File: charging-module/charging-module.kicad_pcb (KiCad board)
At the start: 2 copper layers, 99 x 48 mm, 23 parts, among them IC1 MCP73871-2CCI_ML, J1 OUT, J2 USB_C_Receptacle_USB2.0_16P, J3 BAT

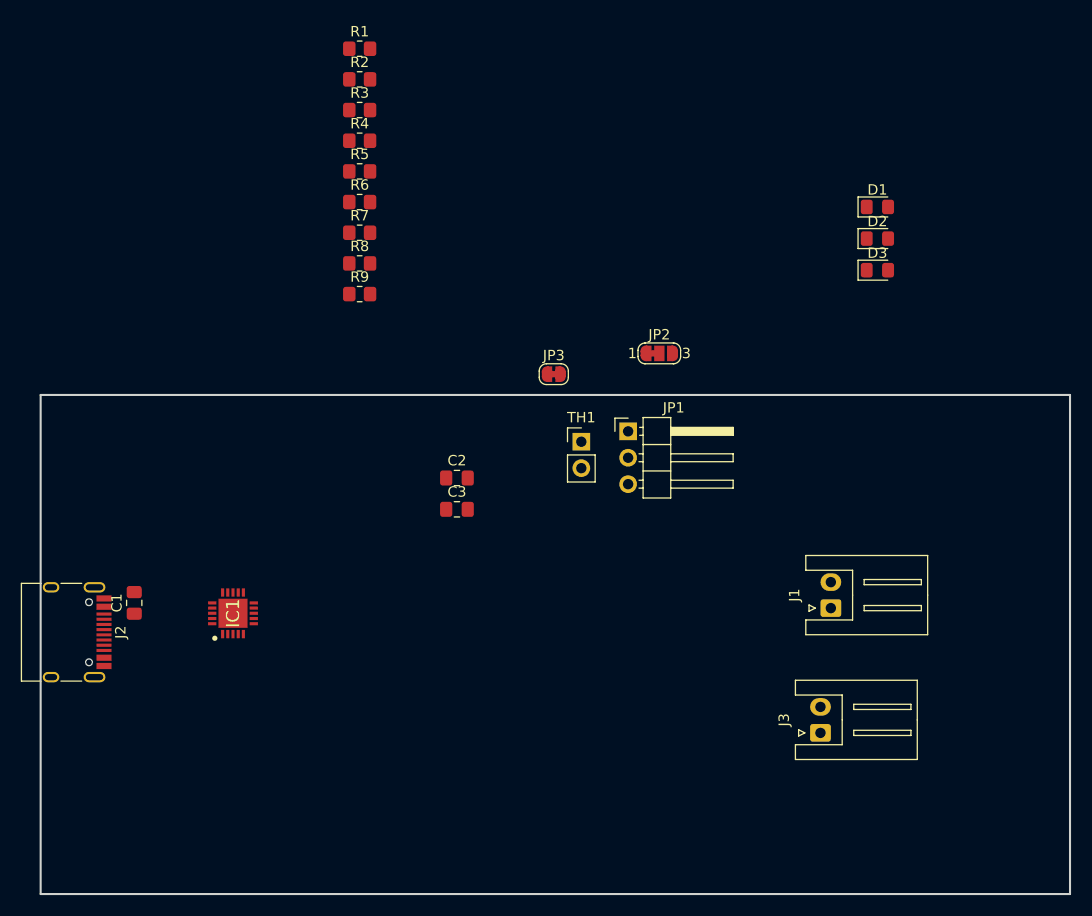
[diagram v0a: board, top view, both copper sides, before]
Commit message: layout
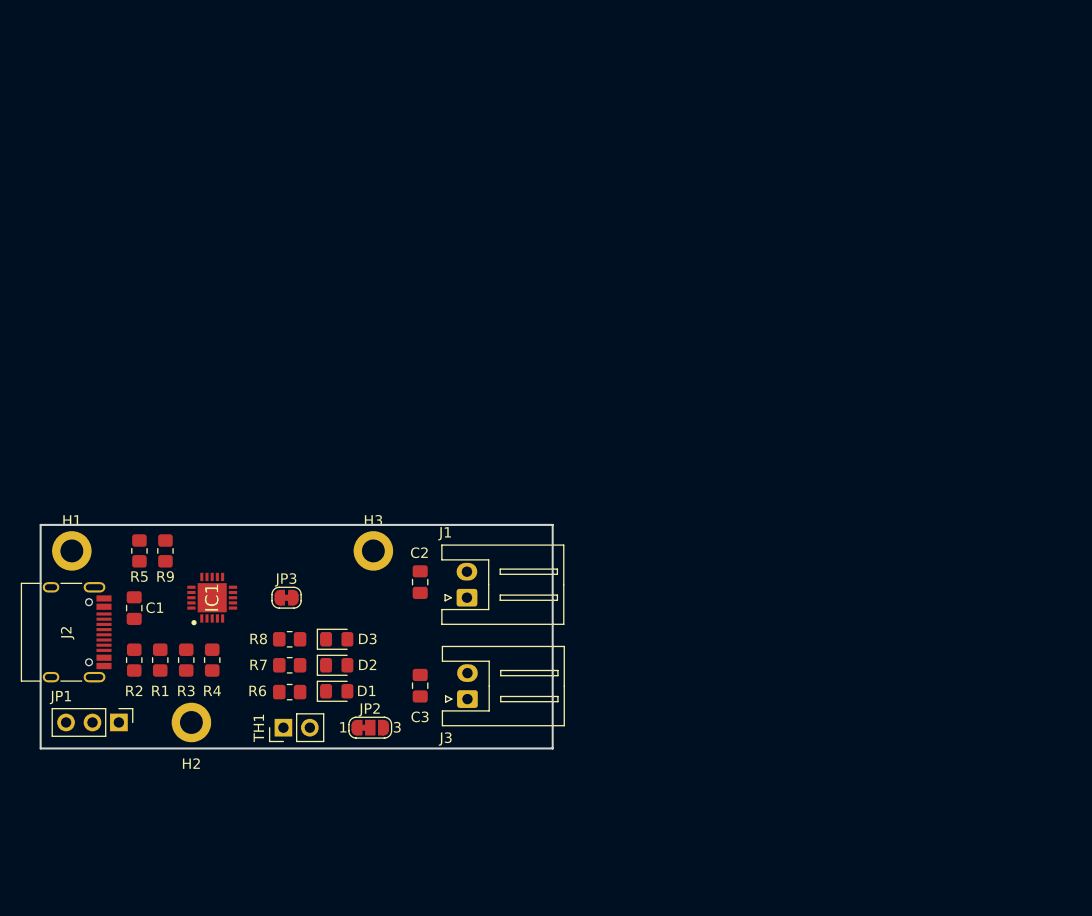
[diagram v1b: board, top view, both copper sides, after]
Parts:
- added H1: MountingHole_Pad, MountingHole:MountingHole_2.2mm_M2_DIN965_Pad, F.Cu at (27.0, 93.0)
- added H2: MountingHole_Pad, MountingHole:MountingHole_2.2mm_M2_DIN965_Pad, F.Cu at (38.5, 109.5)
- added H3: MountingHole_Pad, MountingHole:MountingHole_2.2mm_M2_DIN965_Pad, F.Cu at (56.0, 93.0)
- JP1: footprint Connector_PinHeader_2.54mm:PinHeader_1x03_P2.54mm_Horizontal -> Connector_PinHeader_2.54mm:PinHeader_1x03_P2.54mm_Vertical
- moved D1 69.8 mm to (52.5, 106.5)
- moved D2 66.2 mm to (52.5, 104.0)
- moved D3 63.0 mm to (52.5, 101.5)
- moved R1 61.8 mm to (35.5, 103.5), turned to -90 degrees
- moved R2 59.9 mm to (33.0, 103.5), turned to -90 degrees
- moved JP1 56.4 mm to (31.5, 109.5), turned to -90 degrees
- moved R3 55.5 mm to (38.0, 103.5), turned to -90 degrees
- moved R4 51.9 mm to (40.5, 103.5), turned to -90 degrees
- moved R6 47.6 mm to (48.0, 106.6), turned to 180 degrees
- moved JP2 45.5 mm to (55.7, 110.0)
- moved R5 42.2 mm to (33.5, 93.0), turned to 90 degrees
- moved R7 42.1 mm to (48.0, 104.0), turned to 180 degrees
- moved TH1 39.7 mm to (47.4, 110.0), turned to 90 degrees
- moved R8 36.8 mm to (48.0, 101.5), turned to 180 degrees
- moved J1 35.0 mm to (65.0, 97.5)
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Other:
- board size 99 x 48 mm -> 49.2 x 21.5 mm

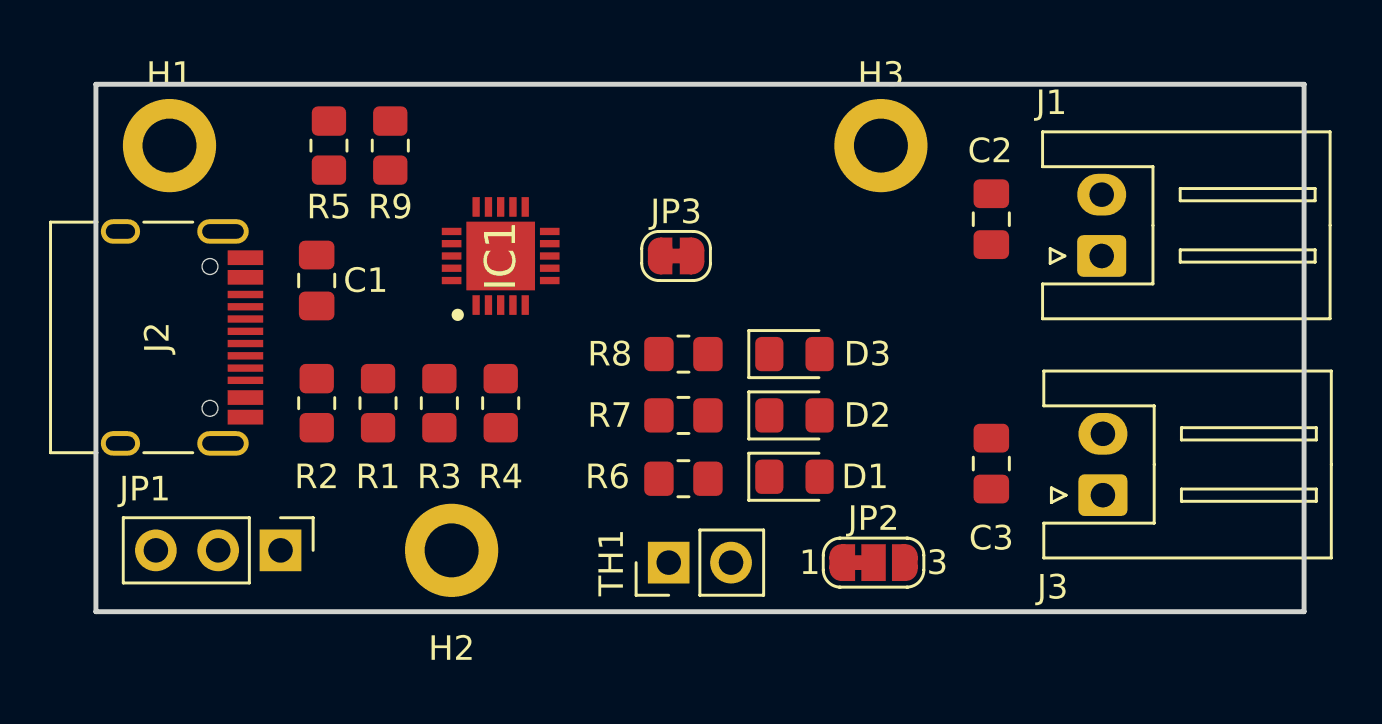
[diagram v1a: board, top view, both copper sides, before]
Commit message: layout done
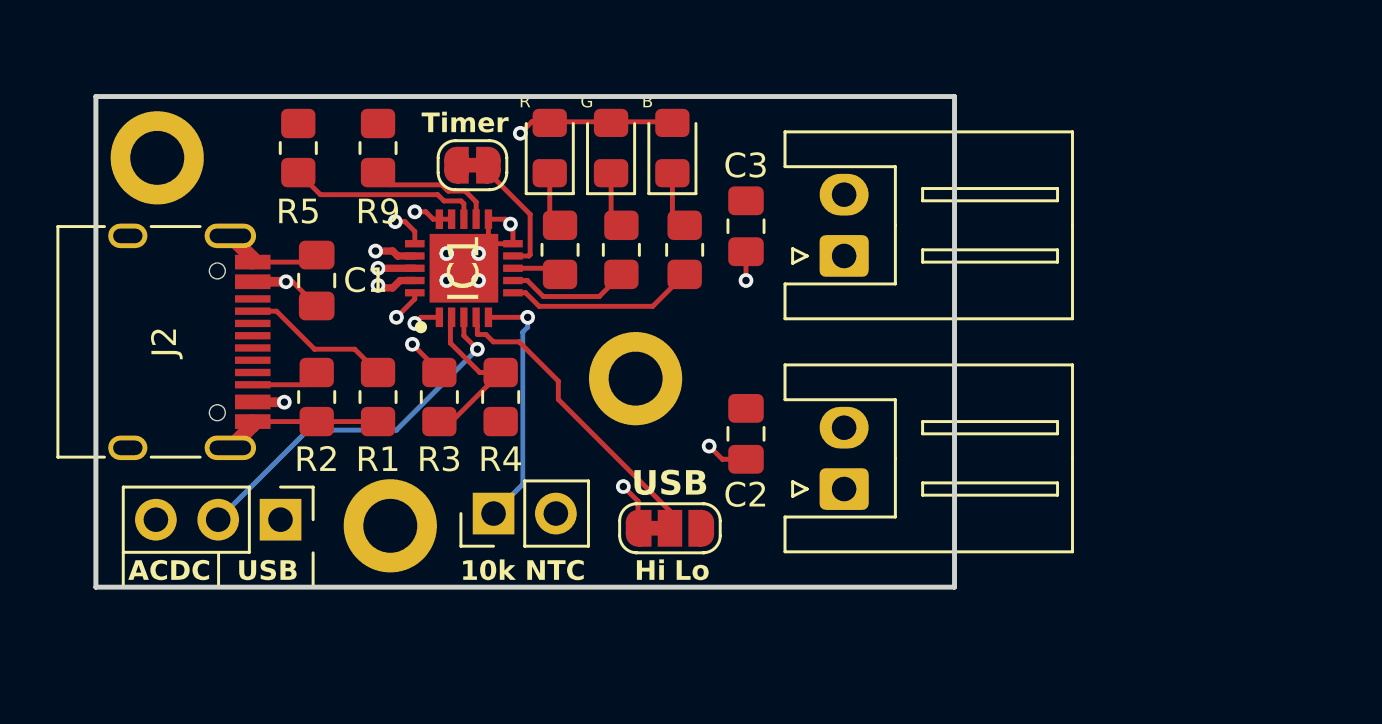
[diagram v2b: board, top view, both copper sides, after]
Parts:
- moved J3 14.4 mm to (54.5, 97.5)
- moved D1 14.3 mm to (47.5, 93.1), turned to 90 degrees
- moved J1 14.2 mm to (54.5, 107.0)
- moved C3 13.9 mm to (50.5, 96.3)
- moved H3 13.8 mm to (46.0, 102.5)
- moved C2 13.3 mm to (50.5, 104.8)
- moved D2 13.2 mm to (45.0, 93.1), turned to 90 degrees
- moved D3 13.0 mm to (42.5, 93.1), turned to 90 degrees
- moved R6 9.33 mm to (48.0, 97.2), turned to -90 degrees
- moved JP3 9.09 mm to (39.4, 93.8), turned to 180 degrees
- moved JP2 8.42 mm to (47.4, 108.6)
- moved TH1 7.41 mm to (40.2, 108.0)
- moved R7 7.21 mm to (45.4, 97.2), turned to -90 degrees
- moved R8 6.59 mm to (42.9, 97.2), turned to -90 degrees
- moved H2 2.69 mm to (36.0, 108.5)
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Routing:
- net /Vin: track 0.00 -> 20.5 mm, vias 0 -> 8
- net GND: track 0.00 -> 16.0 mm, vias 0 -> 5
- net /SEL: track 0.00 -> 15.0 mm, vias 0 -> 1
- net /PROG2: track 0.00 -> 12.7 mm
- net Net-(IC1-THERM): track 0.00 -> 10.2 mm, vias 0 -> 1
- net /PROG1: track 0.00 -> 7.91 mm
- net Net-(IC1-~{PG}): track 0.00 -> 7.77 mm
- net /VPCC: track 0.00 -> 6.95 mm
- net Net-(J2-CC1): track 0.00 -> 6.15 mm
- net /TE: track 0.00 -> 5.20 mm
- net /PROG3: track 0.00 -> 5.20 mm
- net Net-(IC1-STAT2): track 0.00 -> 5.06 mm
- net /Vbat: track 0.00 -> 4.26 mm, vias 0 -> 3
- net /Load: track 0.00 -> 4.14 mm, vias 0 -> 3
- net Net-(J2-CC2): track 0.00 -> 2.82 mm
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- added copper zone on In2.Cu, net /Load
- added copper zone on In2.Cu, net /Vbat
- added copper zone on In1.Cu, net /Vin
- added copper zone on B.Cu, net GND
- added copper zone on F.Cu, net GND
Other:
- board size 49.2 x 21.5 mm -> 35 x 20 mm
- copper layers 2 -> 4
- board text added: "10k NTC"
- board text added: "ACDC"
- board text added: "B"
- board text added: "G"
- board text added: "Hi"
- board text added: "Lo"
- board text added: "R"
- board text added: "Timer"
- board text added: "USB"
